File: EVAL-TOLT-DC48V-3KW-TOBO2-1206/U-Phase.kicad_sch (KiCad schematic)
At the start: 33 parts, among them Q1 IAUS300N10S5N015TATMA1, Q4 IAUS300N10S5N015TATMA1, U3 2EDL8x24G, U4 NL27WZ08USG

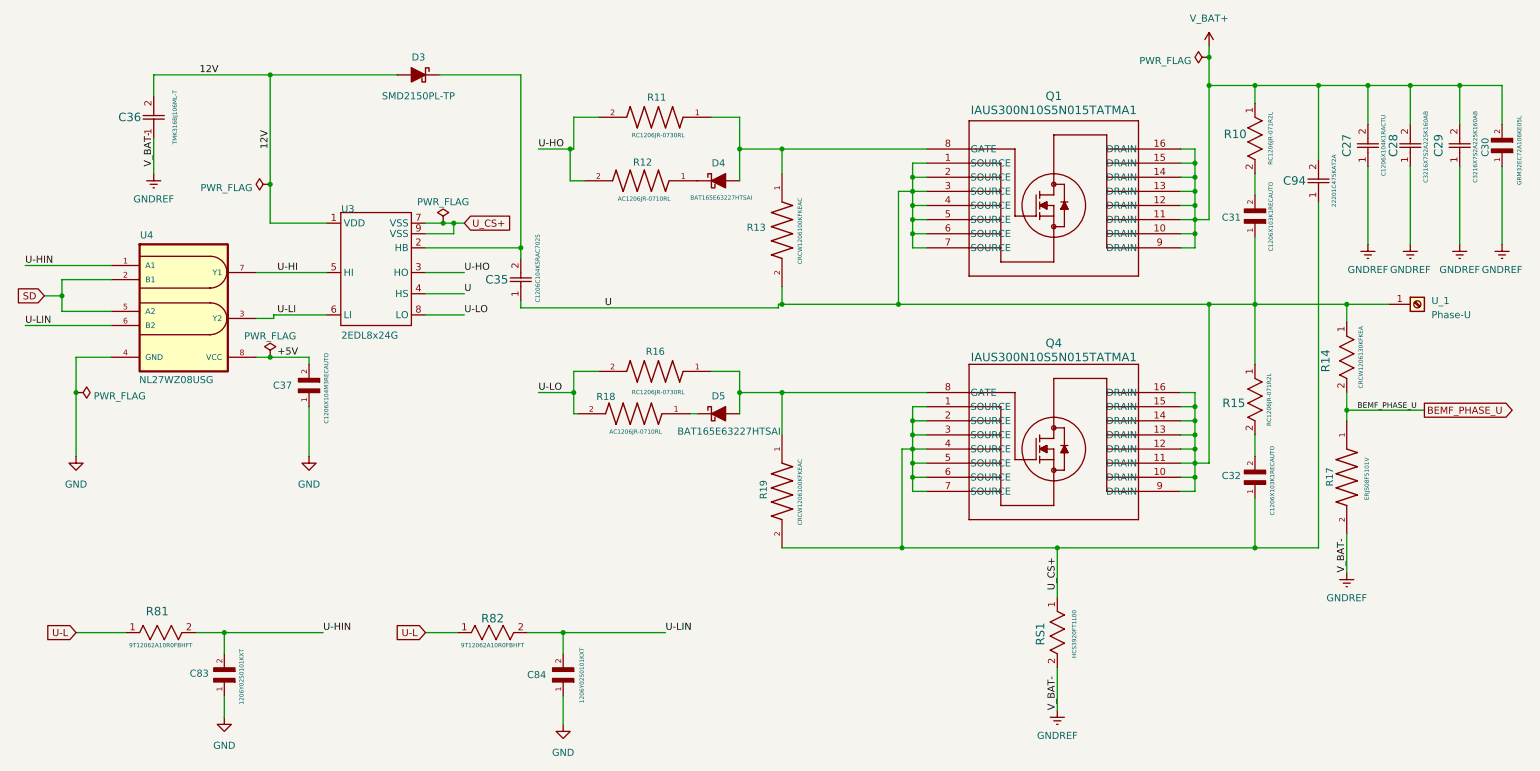
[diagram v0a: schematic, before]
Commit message: v11112024-3
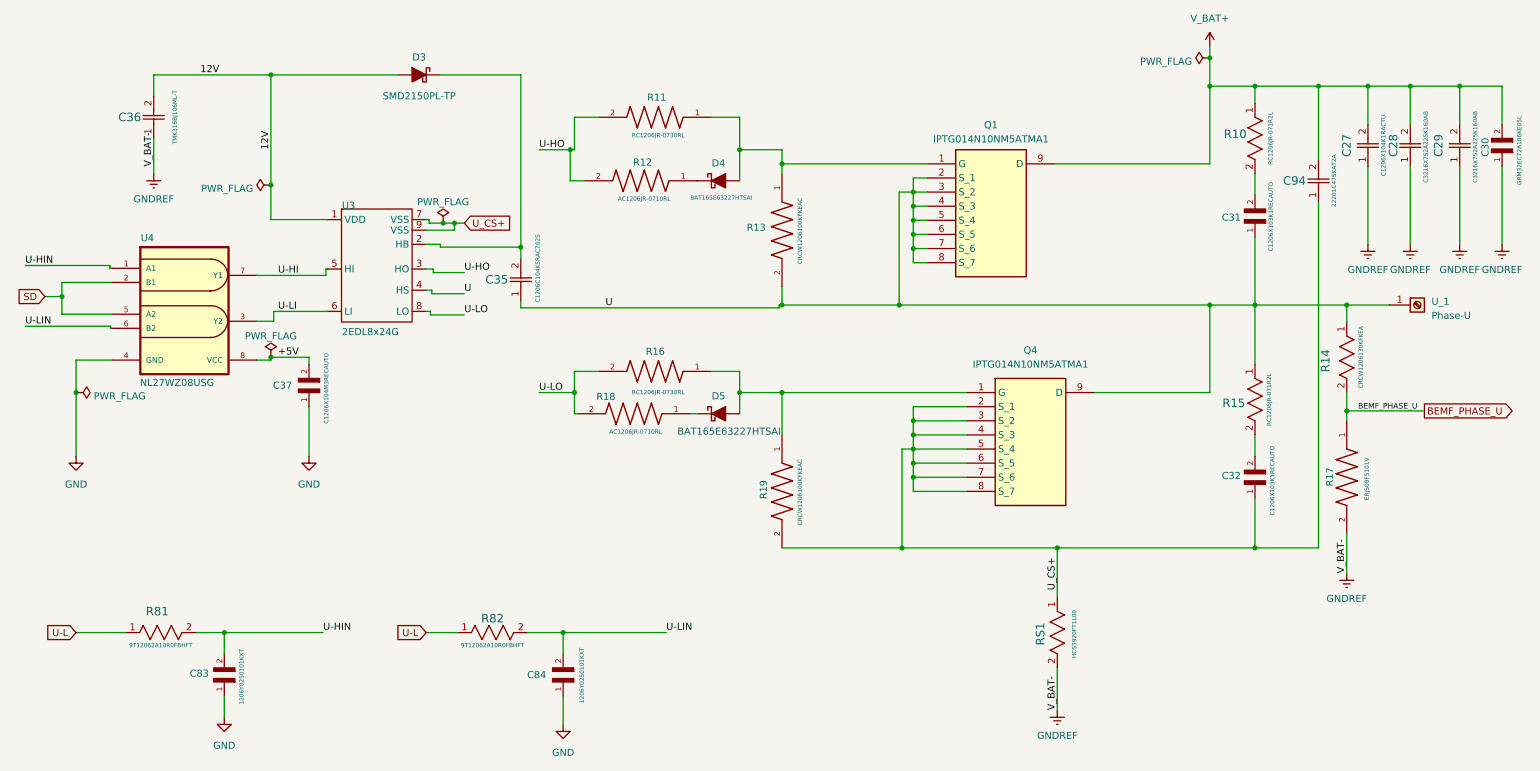
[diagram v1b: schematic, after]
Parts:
- Q1, Q4: value IAUS300N10S5N015TATMA1 -> IPTG014N10NM5ATMA1; footprint just-footprints:Q1 -> Misc-Footprints:IPTG210N25NM3FDATMA1; symbol IAUS300N10S5N015T:IAUS300N10S5N015TATMA1 -> IPTG014N10NM5ATMA1:IPTG014N10NM5ATMA1; Height (none) -> 2.5; Manufacturer_Name (none) -> Infineon; Manufacturer_Part_Number (none) -> IPTG014N10NM5ATMA1; Mouser Part Number (none) -> 726-IPTG014N10NM5ATM; Mouser Price/Stock (none) -> https://www.mouser.co.uk/ProductDetail/Infineon-Technologie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
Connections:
- net U: now also Q1.8 (S_7); no longer Q1.1 (SOURCE), Q4.10 (DRAIN), Q4.11 (DRAIN), Q4.12 (DRAIN), Q4.13 (DRAIN), Q4.14 (DRAIN), Q4.15 (DRAIN), Q4.16 (DRAIN)
- net U_CS+: now also Q4.8 (S_7); no longer Q4.1 (SOURCE)
- net V_BAT+: no longer Q1.10 (DRAIN), Q1.11 (DRAIN), Q1.12 (DRAIN), Q1.13 (DRAIN), Q1.14 (DRAIN), Q1.15 (DRAIN), Q1.16 (DRAIN)
- net at D5.2 (A), R16.1, R19.1: now also Q4.1 (G); no longer Q4.8 (GATE)
- net at D4.2 (A), R11.1, R13.1: now also Q1.1 (G); no longer Q1.8 (GATE)
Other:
- moved on the sheet: U3, U4
